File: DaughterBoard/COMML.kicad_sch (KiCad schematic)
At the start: 25 parts, among them J2 PEC03SAAN, J3 PEC02SAAN, J4 PEC02SAAN

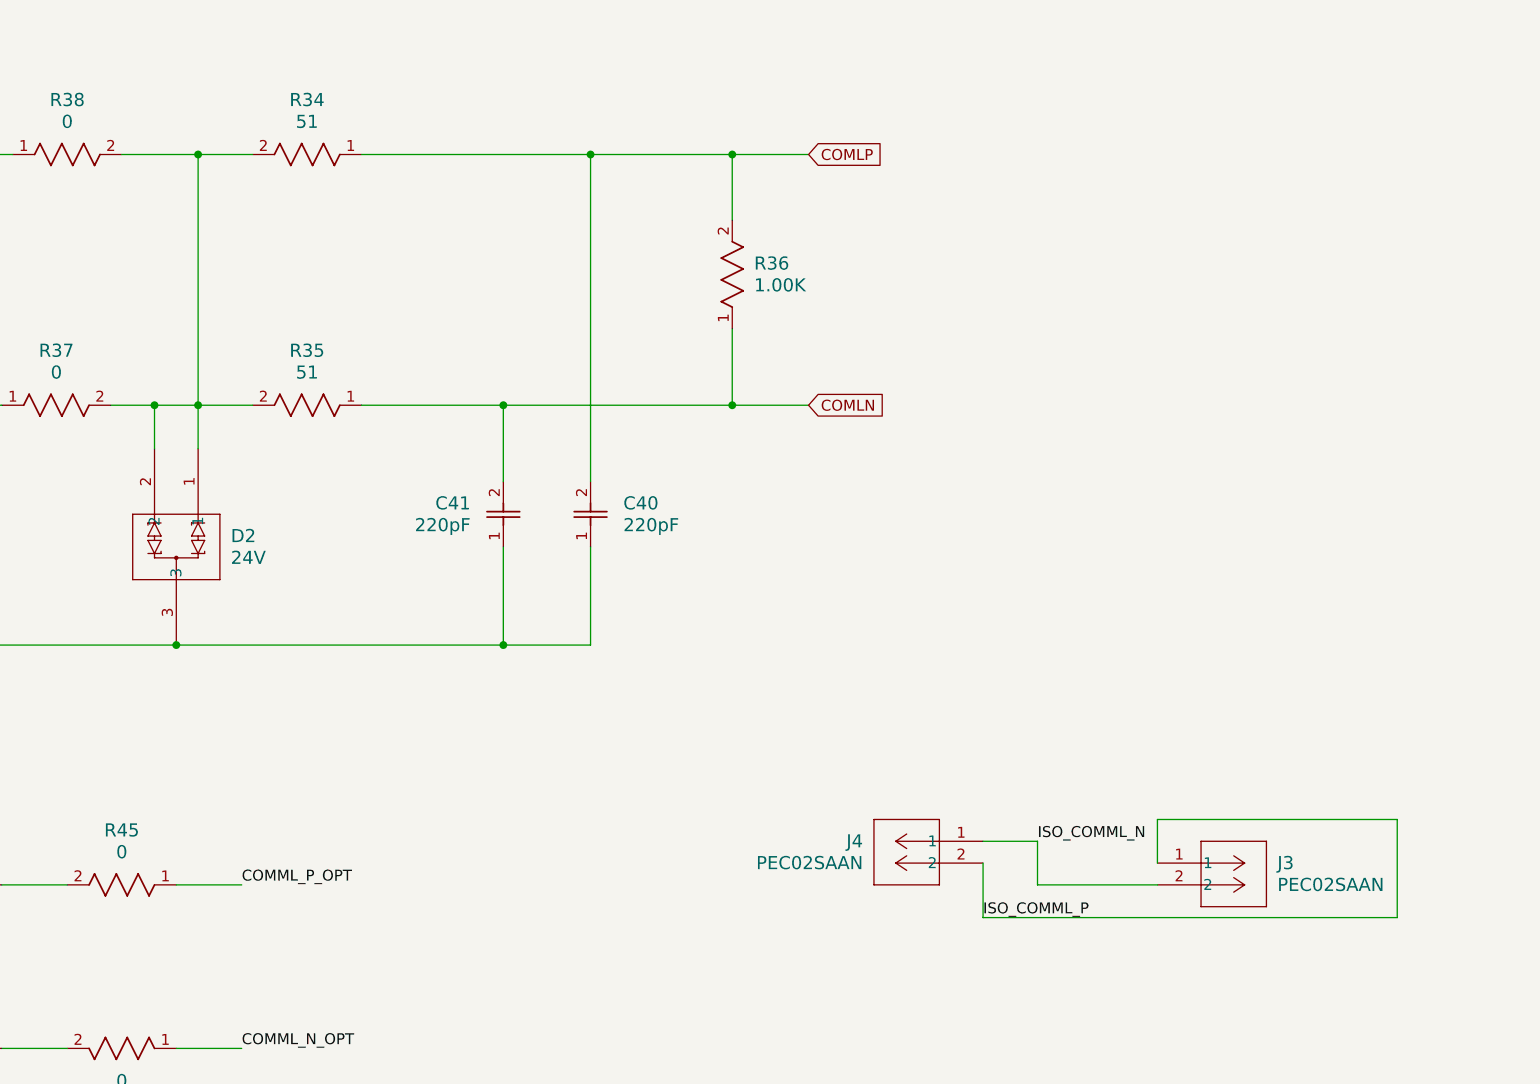
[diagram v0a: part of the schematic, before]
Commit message: Reviewing
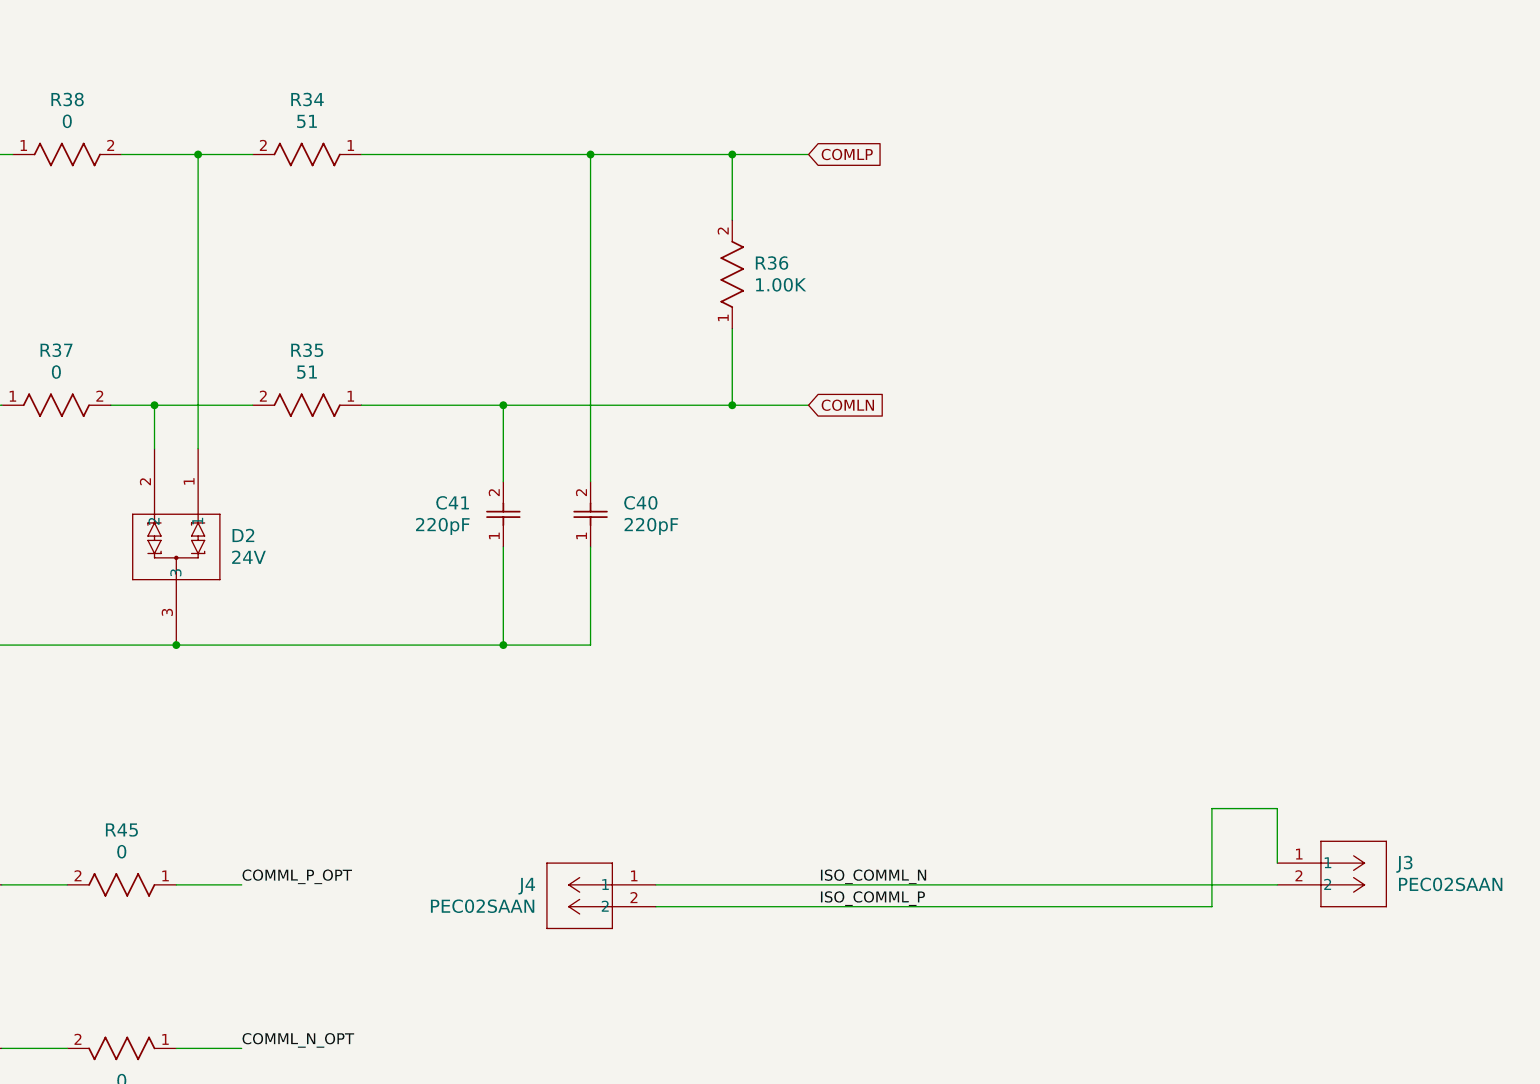
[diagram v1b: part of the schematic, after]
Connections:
- net at D2.2, R35.2, R37.2: no longer D2.1, R34.2, R38.2
- new net: D2.1, R34.2, R38.2
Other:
- moved on the sheet: J3, J4
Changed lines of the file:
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@@
 	(generator "eeschema")
 	(generator_version "8.0")
-	(paper "A4")
+	(paper "A3")
 	(junction
 		(at 193.04 72.39)
@@
 	)
 	(junction
-		(at 130.81 101.6)
-		(diameter 0)
-		(color 0 0 0 0)
-	)
-	(junction
 		(at 88.9 31.75)
 		(diameter 0)
@@
 	(wire
 		(pts
-			(xy 242.57 149.86) (xy 270.51 149.86)
-		)
-		(stroke
-			(width 0)
-			(type default)
-		)
-	)
-	(wire
-		(pts
-			(xy 270.51 161.29) (xy 222.25 161.29)
+			(xy 256.54 148.59) (xy 248.92 148.59)
+		)
+		(stroke
+			(width 0)
+			(type default)
+		)
+	)
+	(wire
+		(pts
+			(xy 184.15 160.02) (xy 248.92 160.02)
 		)
 		(stroke
@@
 	(wire
 		(pts
-			(xy 242.57 154.94) (xy 242.57 149.86)
+			(xy 256.54 154.94) (xy 256.54 148.59)
 		)
 		(stroke
@@
 	(wire
 		(pts
-			(xy 222.25 152.4) (xy 228.6 152.4)
+			(xy 184.15 157.48) (xy 256.54 157.48)
 		)
 		(stroke
@@
 	(wire
 		(pts
-			(xy 228.6 152.4) (xy 228.6 157.48)
-		)
-		(stroke
-			(width 0)
-			(type default)
-		)
-	)
-	(wire
-		(pts
 			(xy 128.27 157.48) (xy 135.89 157.48)
 		)
@@
 	(wire
 		(pts
-			(xy 130.81 106.68) (xy 130.81 101.6)
+			(xy 130.81 72.39) (xy 130.81 106.68)
 		)
 		(stroke
@@
 	(wire
 		(pts
-			(xy 270.51 149.86) (xy 270.51 161.29)
-		)
-		(stroke
-			(width 0)
-			(type default)
-		)
-	)
-	(wire
-		(pts
-			(xy 222.25 161.29) (xy 222.25 154.94)
+			(xy 248.92 148.59) (xy 248.92 160.02)
 		)
 		(stroke
@@
 	(wire
 		(pts
-			(xy 130.81 101.6) (xy 137.16 101.6)
+			(xy 125.73 101.6) (xy 137.16 101.6)
 		)
 		(stroke
@@
 	(wire
 		(pts
-			(xy 228.6 157.48) (xy 242.57 157.48)
-		)
-		(stroke
-			(width 0)
-			(type default)
-		)
-	)
-	(wire
-		(pts
 			(xy 82.55 72.39) (xy 109.22 72.39)
 		)
@@
 	(wire
 		(pts
-			(xy 125.73 101.6) (xy 130.81 101.6)
-		)
-		(stroke
-			(width 0)
-			(type default)
-		)
-	)
-	(wire
-		(pts
 			(xy 128.27 129.54) (xy 166.37 129.54)
 		)
@@
 		(pts
 			(xy 58.42 165.1) (xy 58.42 161.29)
-		)
-		(stroke
-			(width 0)
-			(type default)
-		)
-	)
-	(wire
-		(pts
-			(xy 130.81 72.39) (xy 130.81 101.6)
 		)
 		(stroke
@@
 	)
 	(label "ISO_COMML_N"
-		(at 228.6 152.4 0)
+		(at 203.2 157.48 0)
 		(fields_autoplaced yes)
 		(effects
@@
 	)
 	(label "ISO_COMML_P"
-		(at 222.25 161.29 0)
+		(at 203.2 160.02 0)
 		(fields_autoplaced yes)
 		(effects
@@
 		(lib_name "PEC02SAAN_1")
 		(lib_id "PEC02SAAN:PEC02SAAN")
-		(at 242.57 154.94 0)
+		(at 256.54 154.94 0)
 		(unit 1)
 		(exclude_from_sim no)
@@
 		(fields_autoplaced yes)
 		(property "Reference" "J3"
-			(at 256.54 154.9399 0)
+			(at 270.51 154.9399 0)
 			(effects
 				(font
@@
 		)
 		(property "Value" "PEC02SAAN"
-			(at 256.54 157.4799 0)
+			(at 270.51 157.4799 0)
 			(effects
 				(font
@@
 		)
 		(property "Footprint" "CONN_PxC02S_SUL"
-			(at 242.57 162.306 0)
+			(at 256.54 162.306 0)
 			(effects
 				(font
@@
 		)
 		(property "Datasheet" "PEC02SAAN"
-			(at 243.078 152.654 0)
+			(at 257.048 152.654 0)
 			(effects
 				(font
@@
 		)
 		(property "Description" ""
-			(at 242.57 154.94 0)
+			(at 256.54 154.94 0)
 			(effects
 				(font
@@
 	(symbol
 		(lib_id "PEC02SAAN:PEC02SAAN")
-		(at 222.25 152.4 0)
+		(at 184.15 157.48 0)
 		(mirror y)
 		(unit 1)
@@
 		(dnp no)
 		(property "Reference" "J4"
-			(at 208.28 152.3999 0)
+			(at 170.18 157.4799 0)
 			(effects
 				(font
@@
 		)
 		(property "Value" "PEC02SAAN"
-			(at 208.28 154.9399 0)
+			(at 170.18 160.0199 0)
 			(effects
 				(font
@@
 		)
 		(property "Footprint" "CONN_PxC02S_SUL"
-			(at 223.266 148.59 0)
+			(at 185.166 153.67 0)
 			(effects
 				(font
@@
 		)
 		(property "Datasheet" "PEC02SAAN"
-			(at 222.25 152.4 0)
+			(at 184.15 157.48 0)
 			(effects
 				(font
@@
 		)
 		(property "Description" ""
-			(at 222.25 152.4 0)
-			(effects
-				(font
+			(at 184.15 157.48 0)
+			(effects
+				(font

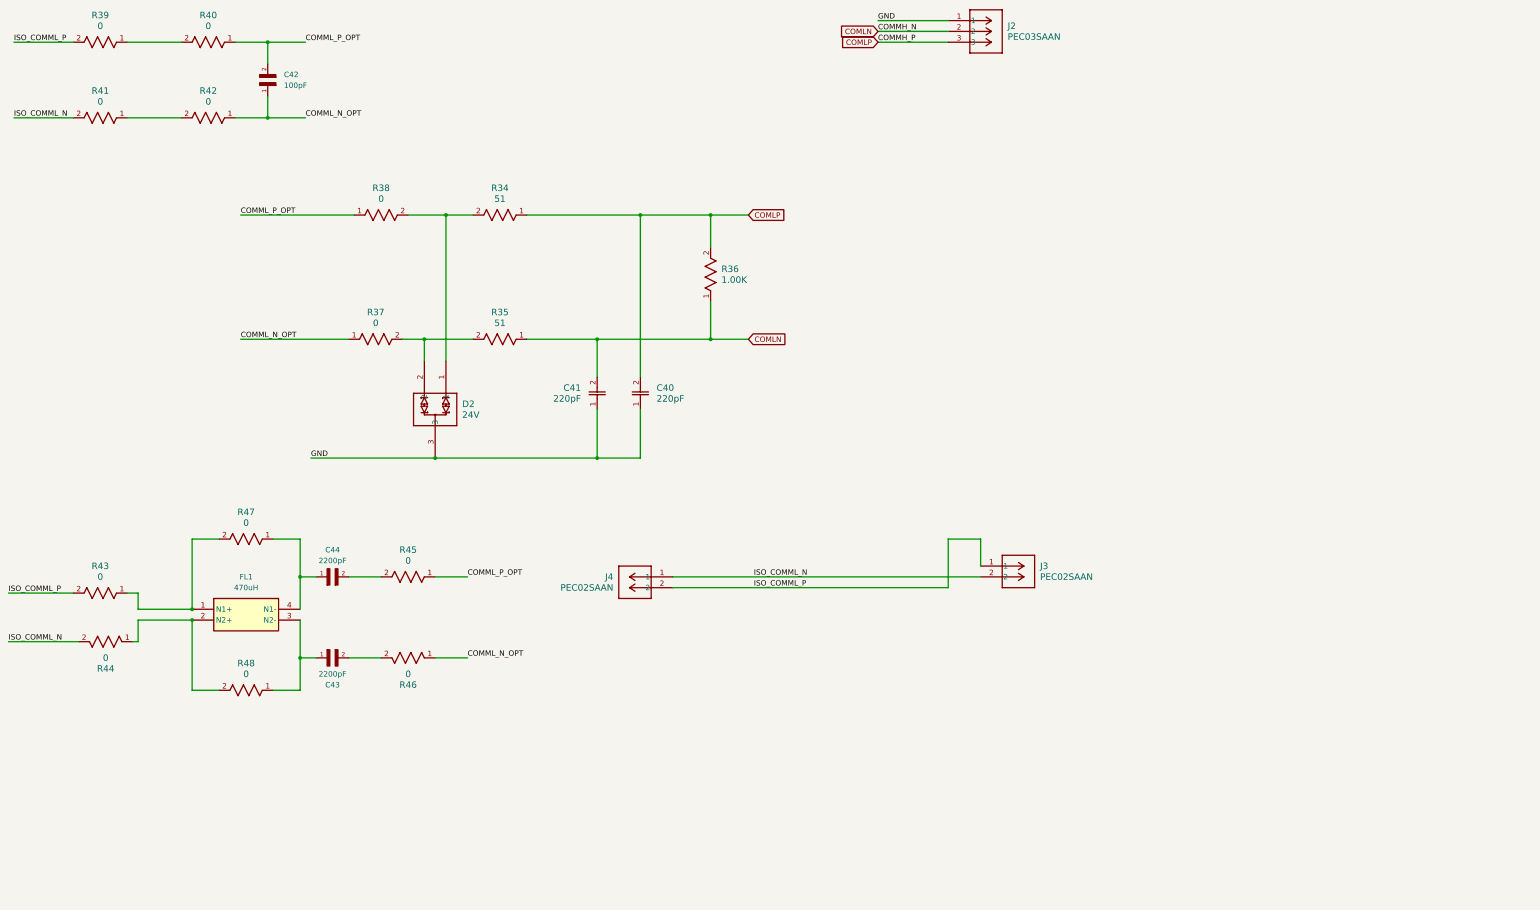
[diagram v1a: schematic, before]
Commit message: ready for pcb
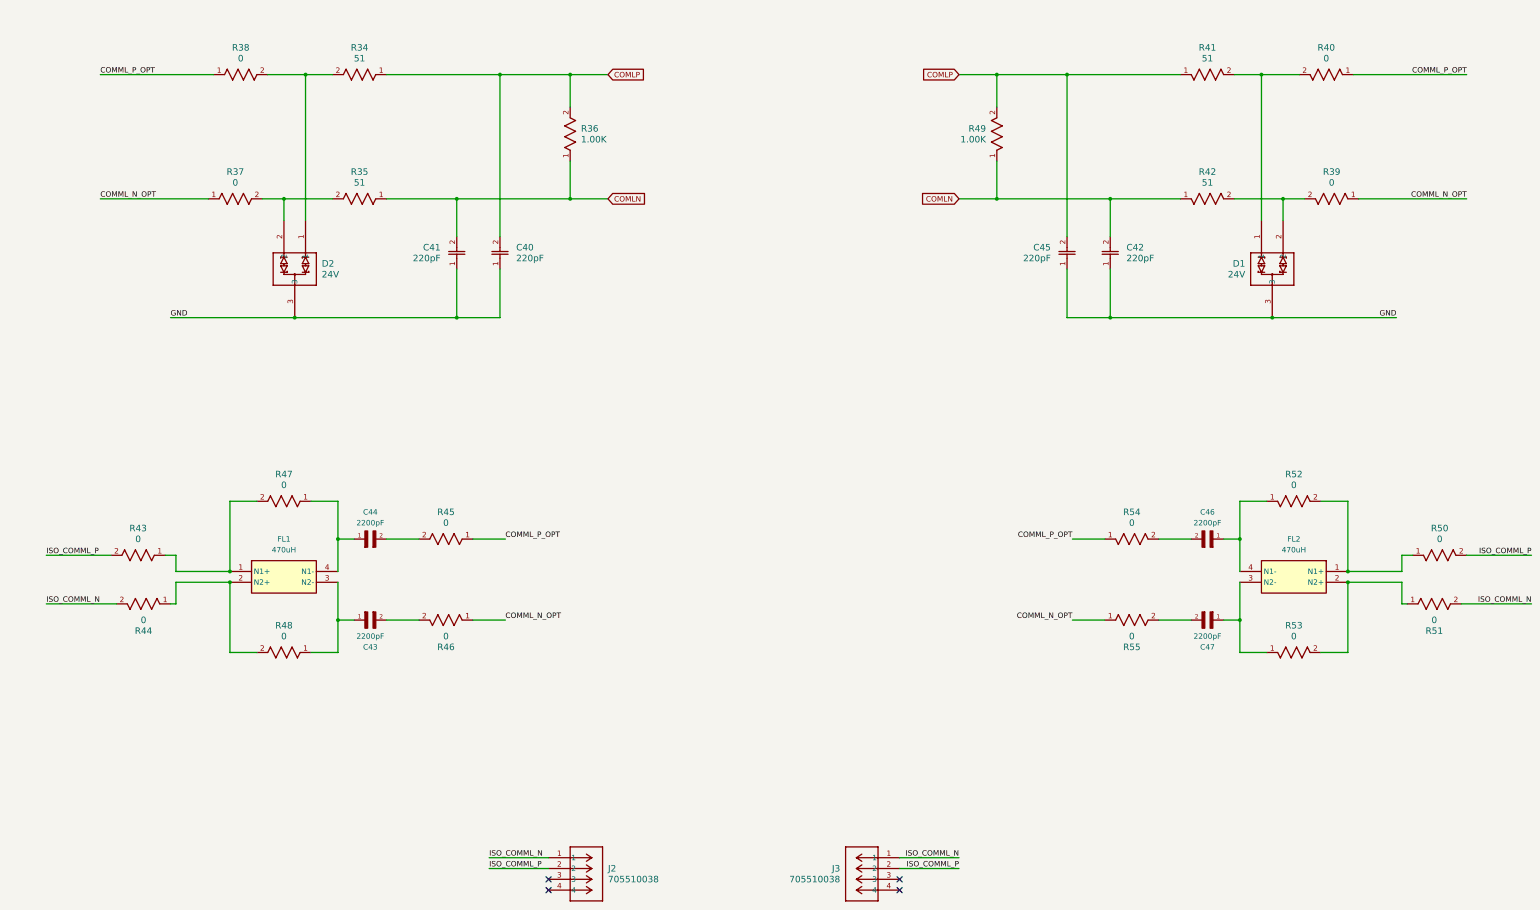
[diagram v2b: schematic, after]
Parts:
- removed C42: 100pF, GCM1885C1H101JA16J:CAPC1608X90N, symbol GCM1885C1H101JA16J:GCM1885C1H101JA16J
- removed J2: PEC03SAAN, CONN_PEC03SAAN_SUL, symbol PEC03SAAN:PEC03SAAN
- removed J3, J4: PEC02SAAN, CONN_PxC02S_SUL, symbol PEC02SAAN:PEC02SAAN
- removed R39, R40, R41, R42: 0, RES_CRCW_0805_VIS, symbol CRCW08050000Z0EAHP:CRCW08050000Z0EAHP
- added C42, C45: 220pF, CAP_CL10_SAM, symbol CL10B221JB8NNNC:CL10B221JB8NNNC
- added C46, C47: 2200pF, 1206J2K00222KXR:CAPC3216X160N, symbol 1206J2K00222KXR:1206J2K00222KXR
- added D1: 24V, SOT23_PESD1_NEX, symbol PESD1CAN,215:PESD1CAN_215
- added FL2: 470uH, 744242471, symbol 744242471:744242471
- added J2, J3: 705510038, CONN_70551-xxxx_04_MOL, symbol 0705510038:705510038
- added R39, R40: 0, RC0603N_YAG, symbol RC0603JR-070RL:RC0603JR-070RL
- added R41, R42: 51, RC0603N_VIS, symbol CRCW060351R0JNEA:CRCW060351R0JNEA
- added R49: 1.00K, RC0603N_PAN, symbol ERJ-3EKF1001V:ERJ-3EKF1001V
- added R50, R51, R52, R53, R54, R55: 0, RES_CRCW_0805_VIS, symbol CRCW08050000Z0EAHP:CRCW08050000Z0EAHP
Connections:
- net COMLN: now also C42.2, R42.1, R49.1
- net COMLP: now also C45.2, R41.1, R49.2
- net COMML_N_OPT: now also R39.1, R55.1
- net COMML_P_OPT: now also R40.1, R54.1
- net GND: now also C42.1, C45.1, D1.3
- net ISO_COMML_N: now also J2.1, J3.1, R51.2
- net ISO_COMML_P: now also J2.2, J3.2, R50.2
- new net: C47.2, R55.2
- new net: D1.1, R40.2, R41.2
- new net: D1.2, R39.2, R42.2
- new net: C47.1, FL2.3 (N2-), R53.1
- new net: FL2.2 (N2+), R51.1, R53.2
- new net: C46.1, FL2.4 (N1-), R52.1
- new net: FL2.1 (N1+), R50.1, R52.2
- new net: C46.2, R54.2
- no-connect marks 0 -> 4
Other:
- moved on the sheet: C40, C41, C43, C44, D2, FL1, R34, R35, R36, R37, R38, R43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
